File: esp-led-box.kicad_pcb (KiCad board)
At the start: 2 copper layers, 40 x 65 mm, 46 parts, among them J1 Conn_01x03, J2 Conn_01x03_Female, J3 Conn_01x02_Female, J4 USB_B_Micro, Q1 BSS138, SW3 SW_SPDT, U1 MP2307, U2 LM3940, U3 ESP-12F

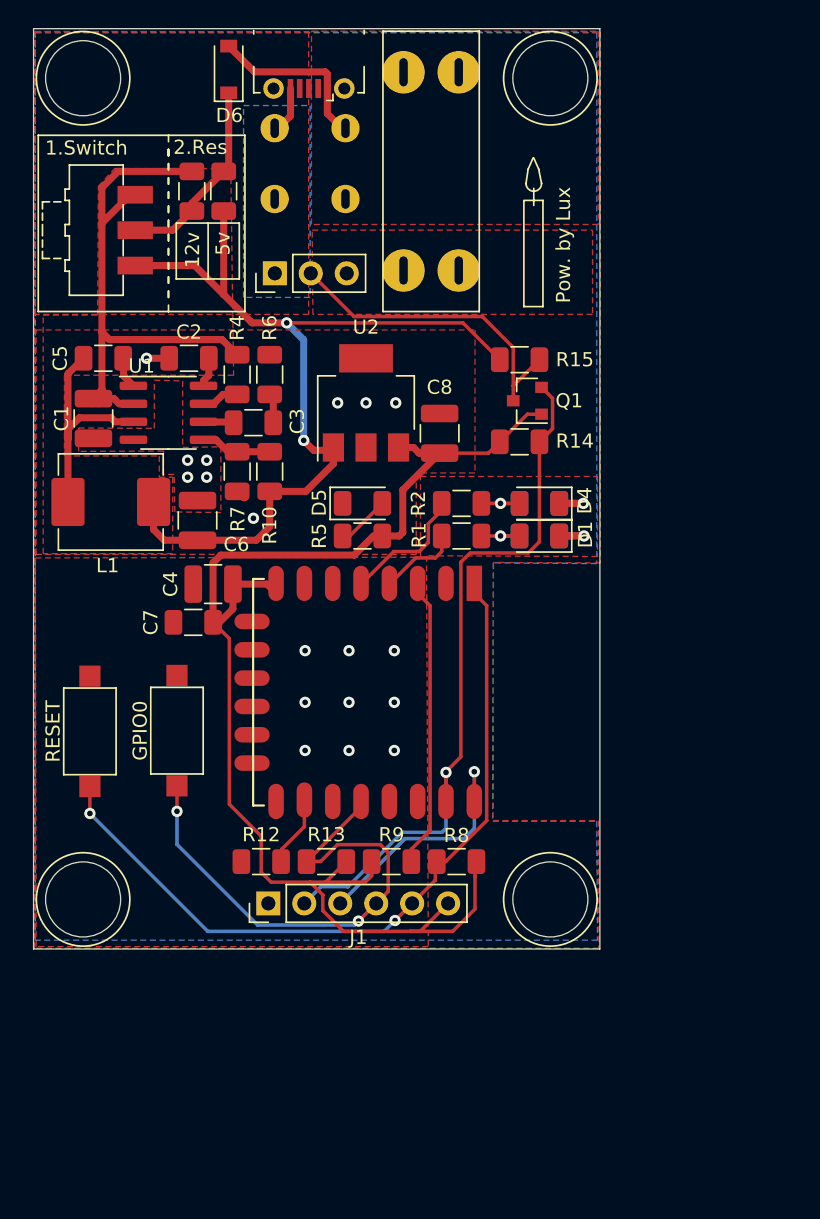
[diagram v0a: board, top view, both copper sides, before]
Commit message: my new version is coming
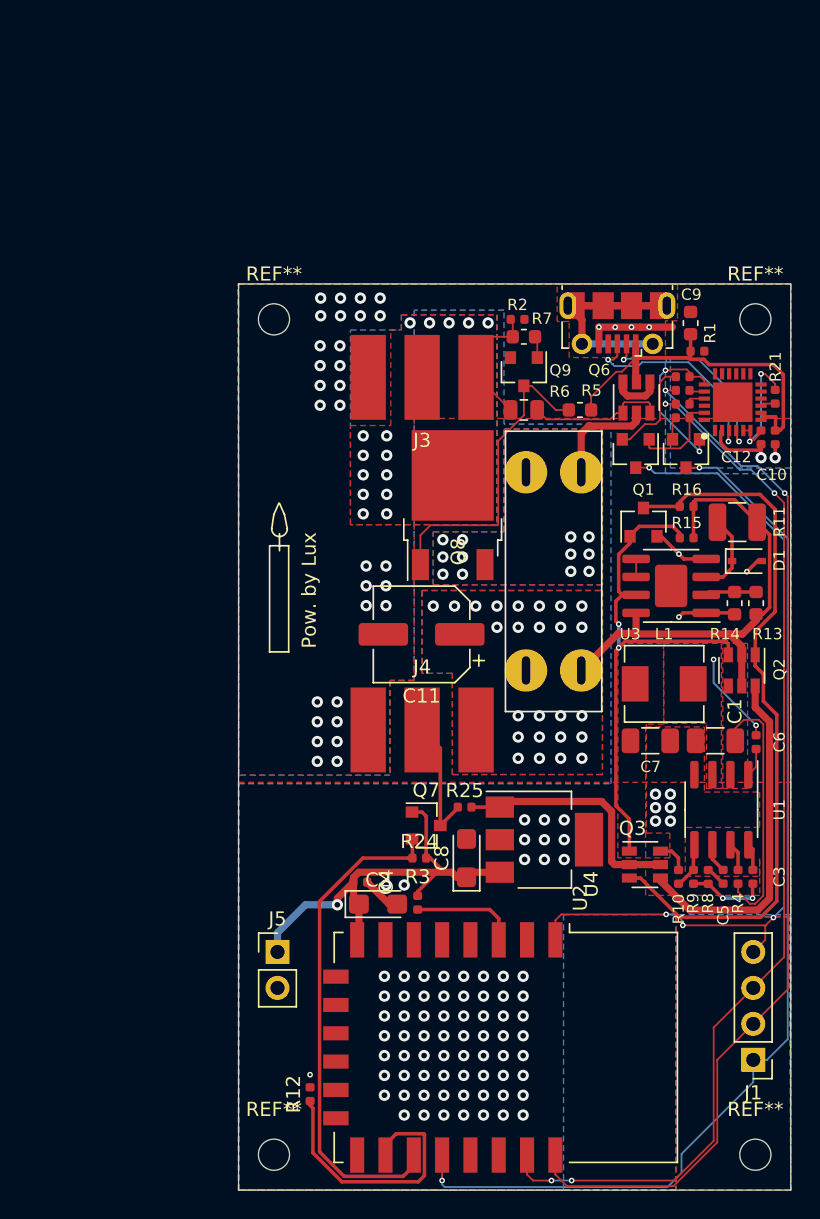
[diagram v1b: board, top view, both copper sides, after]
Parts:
- removed D2, D3, D4, D5: LED, LED_SMD:LED_1206_3216Metric
- removed D6: D, Diode_SMD:D_SOD-123
- removed GPIO0, RESET: SW_Push, Button_Switch_SMD:SW_SPST_CK_RS282G05A3
- removed the REF** at (147.5, 101.5)
- removed the REF** at (147.5, 43.5)
- removed the REF** at (114.5, 101.5)
- removed the REF** at (114.5, 43.5)
- removed SW3: SW_SPDT, Button_Switch_SMD:SW_SPDT_CK-JS102011SAQN
- added C10: 1uF, Capacitor_SMD:C_0402_1005Metric, F.Cu at (163.4, 68.8)
- added C11: 220u, Capacitor_SMD:CP_Elec_6.3x7.7, F.Cu at (138.4, 82.8)
- added C12: 100nF, Capacitor_SMD:C_0402_1005Metric, F.Cu at (162.4, 68.8)
- added C9: 10u, Capacitor_SMD:C_0603_1608Metric, F.Cu at (157.4, 60.8)
- added IC1: CP2105-F01-GMR, CP2105-F01-GMR:QFN50P400X400X80-25N-D, F.Cu at (160.4, 66.3)
- added J5: Conn_01x02, Connector_PinHeader_2.54mm:PinHeader_1x02_P2.54mm_Vertical, F.Cu at (128.2, 105.2)
- added Q2: Q_PMOS_DGS, Package_TO_SOT_SMD:SOT-23-6, F.Cu at (161.0, 85.3)
- added Q3: Q_PMOS_DGS, Package_TO_SOT_SMD:SOT-23-6, F.Cu at (154.2, 99.0)
- added Q4: S8050, Package_TO_SOT_SMD:SOT-23, F.Cu at (157.1, 70.0)
- added Q5: S8050, Package_TO_SOT_SMD:SOT-23, F.Cu at (153.6, 70.0)
- added Q6: Q_PMOS_DGS, Package_TO_SOT_SMD:SOT-23-6, F.Cu at (153.6, 66.0)
- added Q7: BSS138, Package_TO_SOT_SMD:SOT-23, F.Cu at (138.8, 96.2)
- added Q8: Q_PMOS_DGS, Package_TO_SOT_SMD:TO-252-2, F.Cu at (140.6, 73.6)
- added Q9: Q_NMOS, Package_TO_SOT_SMD:SOT-23, F.Cu at (145.7, 64.2)
- added R16: 20K, Resistor_SMD:R_0402_1005Metric, F.Cu at (157.1, 73.7)
- added R17: 12K, Resistor_SMD:R_0402_1005Metric, F.Cu at (156.9, 67.4)
- added R18: 12K, Resistor_SMD:R_0402_1005Metric, F.Cu at (156.9, 64.5)
- added R21: 4.7K, Resistor_SMD:R_0402_1005Metric, F.Cu at (163.4, 66.0)
- added R22: 300, Resistor_SMD:R_0402_1005Metric, F.Cu at (156.9, 66.5)
- added R23: 300, Resistor_SMD:R_0402_1005Metric, F.Cu at (156.9, 65.5)
- added R24: 10K, Resistor_SMD:R_0402_1005Metric, F.Cu at (138.3, 98.5)
- added R25: 10K, Resistor_SMD:R_0402_1005Metric, F.Cu at (141.5, 95.0)
- added REF**: MountingHole_2.2mm_M2, MountingHole:MountingHole_2.2mm_M2, F.Cu at (162.0, 60.5)
- added REF**: MountingHole_2.2mm_M2, MountingHole:MountingHole_2.2mm_M2, F.Cu at (128.0, 60.5)
- added REF**: MountingHole_2.2mm_M2, MountingHole:MountingHole_2.2mm_M2, F.Cu at (128.0, 119.5)
- added REF**: MountingHole_2.2mm_M2, MountingHole:MountingHole_2.2mm_M2, F.Cu at (162.0, 119.5)
- added U4: LM3940, Package_TO_SOT_SMD:SOT-223-3_TabPin2, F.Cu at (147.1, 97.2)
- C1: value 10uF/25V -> 10u/25V; footprint Capacitor_SMD:C_1210_3225Metric -> Capacitor_SMD:C_1206_3216Metric
- C2: value 0.1uF -> 10uF; footprint Capacitor_SMD:C_1206_3216Metric -> Capacitor_Tantalum_SMD:CP_EIA-3216-18_Kemet-A
- C3: value 3.9nF -> 100nF; footprint Capacitor_SMD:C_1206_3216Metric -> Capacitor_SMD:C_0402_1005Metric
- C4: value 10uF -> 100nF; footprint Capacitor_SMD:C_1210_3225Metric -> Capacitor_SMD:C_0402_1005Metric
- C5: value 10nF -> 3.9nF; footprint Capacitor_SMD:C_1206_3216Metric -> Capacitor_SMD:C_0402_1005Metric
- C6: value 22uF/6.3V -> 10nF; footprint Capacitor_SMD:C_1210_3225Metric -> Capacitor_SMD:C_0402_1005Metric
- C7: value 100nF -> 47uF/6.3V
- C8: footprint Capacitor_SMD:C_1210_3225Metric -> Capacitor_Tantalum_SMD:CP_EIA-3216-18_Kemet-A
- D1: value LED -> 2.4V; footprint LED_SMD:LED_1206_3216Metric -> Diode_SMD:D_SOD-323
- J1: value Conn_01x03 -> Conn_01x04; footprint Connector_PinHeader_2.54mm:PinHeader_1x06_P2.54mm_Vertical -> Connector_PinHeader_2.54mm:PinHeader_1x04_P2.54mm_Vertical
- J2: value Conn_01x03_Female -> USB_B_Micro; footprint Connector_PinHeader_2.54mm:PinHeader_1x03_P2.54mm_Vertical -> Connector_USB:USB_Micro-B_Molex-105017-0001
- J3: value Conn_01x02_Female -> Conn_01x03_Female; footprint esp-light-box:WG235-2P -> esp-light-box:SolderWire_1x03_2.5x6; moved to F.Cu
- J4: value USB_B_Micro -> Conn_01x03_Female; footprint Connector_USB:USB_Micro-B_Molex-105017-0001 -> esp-light-box:SolderWire_1x03_2.5x6
- L1: footprint Inductor_SMD:L_Abracon_ASPI-0630LR -> Inductor_SMD:L_Sunlord_MWSA0518_5.4x5.2mm
- Q1: value BSS138 -> Q_NMOS
- R1, R2: value 120 -> 1M; footprint Resistor_SMD:R_1206_3216Metric -> Resistor_SMD:R_0402_1005Metric
- R10, R12, R4: footprint Resistor_SMD:R_1206_3216Metric -> Resistor_SMD:R_0402_1005Metric
- R11: value 0 -> 360; footprint Resistor_SMD:R_1206_3216Metric -> Resistor_SMD:R_1210_3225Metric
- R13: value 10K -> 24K; footprint Resistor_SMD:R_1206_3216Metric -> Resistor_SMD:R_0603_1608Metric
- R14: footprint Resistor_SMD:R_1206_3216Metric -> Resistor_SMD:R_0603_1608Metric
- R15: value 10K -> 20K; footprint Resistor_SMD:R_1206_3216Metric -> Resistor_SMD:R_0402_1005Metric
- R3: value 0 -> 10K; footprint Resistor_SMD:R_1206_3216Metric -> Resistor_SMD:R_0402_1005Metric
- R5: value 120 -> 20K; footprint Resistor_SMD:R_1206_3216Metric -> Resistor_SMD:R_0603_1608Metric
- R6: value 6.8K -> 300; footprint Resistor_SMD:R_1206_3216Metric -> Resistor_SMD:R_0805_2012Metric
- R7: value 10K/1% -> 20K; footprint Resistor_SMD:R_1206_3216Metric -> Resistor_SMD:R_0603_1608Metric
- R8: value 10K -> 6.8K; footprint Resistor_SMD:R_1206_3216Metric -> Resistor_SMD:R_0402_1005Metric
- R9: value 10K -> 10K/1%; footprint Resistor_SMD:R_1206_3216Metric -> Resistor_SMD:R_0402_1005Metric
- U2: value LM3940 -> ESP-12F; footprint Package_TO_SOT_SMD:SOT-223-3_TabPin2 -> RF_Module:ESP-12E
- U3: value ESP-12F -> LM211; footprint ESP8266:ESP-12E -> Package_SO:SOIC-8-1EP_3.9x4.9mm_P1.27mm_EP2.29x3mm
- moved C5 57.1 mm to (159.7, 99.9), turned to 270 degrees
- moved R3 52.7 mm to (138.2, 101.7), turned to 270 degrees
- moved R4 50.1 mm to (160.8, 99.9), turned to 90 degrees
- moved C1 49.5 mm to (159.2, 90.3), turned to 180 degrees
- moved U1 48.1 mm to (159.6, 95.1), turned to 270 degrees
- moved C3 47.7 mm to (161.8, 99.9), turned to 270 degrees
- moved J4 47.4 mm to (138.5, 89.5), turned to 0 degrees
- moved U2 46.6 mm to (144.4, 111.9), turned to 270 degrees
- moved R11 43.2 mm to (160.7, 74.8), turned to 0 degrees
- moved C6 42.4 mm to (162.1, 90.4), turned to 270 degrees
- moved L1 41.1 mm to (155.6, 86.2), turned to 180 degrees
- moved C2 40.8 mm to (135.3, 101.8), turned to 0 degrees
- moved R10 40.7 mm to (156.6, 99.9), turned to 270 degrees
- moved J1 36.0 mm to (161.8, 112.8), turned to 180 degrees
- moved R13 35.4 mm to (162.1, 80.5), turned to 90 degrees
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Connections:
- C2 pad 1: Net-(C2-Pad1) -> +3V3
- C3 pad 2: Net-(C3-Pad2) -> GND
- C6 pad 1: +5V -> Net-(C6-Pad1)
- C6 pad 2: GND -> Net-(C6-Pad2)
- C7 pad 1: +3V3 -> /BUCK_5V
- D1 pad 1: GND -> Net-(D1-Pad1)
- D1 pad 2: Net-(D1-Pad2) -> GND
- F1 pad 1: Net-(F1-Pad1) -> /DC_VDD
- F1 pad 2: VSS -> VDD
- J1 pad 1: GND -> /GPIO0
- J1 pad 2: /RXD|CONTROL -> /TXD
- J1 pad 3: /TXD -> /RXD
- J1 pad 4: /GPIO0 -> /RESET
- J2 pad 1: GND -> VBUS
- J2 pad 2: Net-(J2-Pad2) -> /D-
- J2 pad 3: Net-(F1-Pad1) -> /D+
- J3 pad 1: GND -> VDC
- J3 pad 2: VSS -> VDC
- J4 pad 1: VSS -> GND
- J4 pad 3: Net-(J4-Pad3) -> VDD
- L1 pad 1: Net-(C5-Pad1) -> Net-(C6-Pad1)
- L1 pad 2: +5V -> /BUCK_5V
- Q1 pad 1: +3V3 -> /~12V_SEL
- Q1 pad 2: /RXD|CONTROL -> GND
- Q1 pad 3: Net-(J2-Pad2) -> /~5V_SEL
- R1 pad 1: /GREEN_LED -> VBUS
- R1 pad 2: Net-(D1-Pad2) -> GND
- R10 pad 1: +5V -> /BUCK_5V
- R11 pad 1: +VDC -> Net-(D1-Pad1)
- R11 pad 2: +5V -> VDD
- R12 pad 1: GND -> Net-(R12-Pad1)
- R12 pad 2: Net-(R12-Pad2) -> GND
- R13 pad 1: +3V3 -> VDD
- R13 pad 2: /GPIO0 -> Net-(R13-Pad2)
- R14 pad 1: /RXD|CONTROL -> Net-(R13-Pad2)
- R14 pad 2: +3V3 -> GND
- R15 pad 1: Net-(J2-Pad2) -> VDD
- R15 pad 2: +5V -> /~12V_SEL
- R2 pad 1: /RED_LED -> VDC
- R2 pad 2: Net-(D3-Pad2) -> GND
- R3 pad 1: +VDC -> +3V3
- R3 pad 2: +12V -> Net-(R3-Pad2)
- R5 pad 1: +3V3 -> VBUS
- R5 pad 2: Net-(D5-Pad2) -> /~VDC_SEL
- R6 pad 1: Net-(C3-Pad2) -> VDC
- R6 pad 2: GND -> /VDC_ON
- R7 pad 1: Net-(R10-Pad2) -> VDC
- R7 pad 2: GND -> Net-(Q9-Pad1)
- R8 pad 1: /RESET -> Net-(C5-Pad2)
- R8 pad 2: +3V3 -> GND
- R9 pad 1: Net-(R9-Pad1) -> Net-(R10-Pad2)
- R9 pad 2: +3V3 -> GND
- U1 pad 1: Net-(C5-Pad2) -> Net-(C6-Pad2)
- U1 pad 3: Net-(C5-Pad1) -> Net-(C6-Pad1)
- U1 pad 6: Net-(C3-Pad1) -> Net-(C5-Pad1)
- U1 pad 8: Net-(C2-Pad1) -> Net-(C3-Pad1)
- U2 pad 1: +5V -> /RESET
- U2 pad 2: GND -> Net-(U2-Pad2)
- U2 pad 3: +3V3 -> Net-(R3-Pad2)
- U3 pad 1: /RESET -> GND
- U3 pad 2: Net-(U3-Pad2) -> Net-(R13-Pad2)
- U3 pad 3: Net-(R9-Pad1) -> Net-(D1-Pad1)
- U3 pad 4: /GREEN_LED -> GND
- U3 pad 5: /RED_LED -> Net-(U3-Pad5)
- U3 pad 6: Net-(U3-Pad6) -> Net-(U3-Pad5)
- U3 pad 7: Net-(U3-Pad7) -> /~12V_SEL
- U3 pad 8: +3V3 -> VDD
- U3 pad 9: GND -> (no net)
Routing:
- net /RXD: track 0.00 -> 76.9 mm, vias 0 -> 4
- net +3V3: track 95.5 -> 33.5 mm, vias 0 -> 1
- net /TXD: track 17.1 -> 74.6 mm, vias 1 -> 2
- net /RXD|CONTROL: track 52.2 -> 0.00 mm, vias 1 -> 0
- net /~5V_SEL: track 0.00 -> 51.2 mm
- net +5V: track 65.5 -> 17.4 mm, vias 2 -> 0
- net /GPIO0: track 39.3 -> 77.2 mm
- net /~12V_SEL: track 0.00 -> 37.5 mm, vias 0 -> 2
- net /LED_CTRL: track 0.00 -> 35.3 mm
- net VDD: track 0.00 -> 35.2 mm, vias 0 -> 25
- net VBUS: track 0.00 -> 30.4 mm
- net /DC_5V: track 0.00 -> 24.5 mm
- net Net-(J2-Pad2): track 22.8 -> 0.00 mm
- net +12V: track 40.9 -> 18.3 mm
- net /~VDC_SEL: track 0.00 -> 22.3 mm
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- added copper zone on B.Cu, net (none)
- added copper zone on F.Cu, net +12V
- added copper zone on F.Cu, net /BUCK_5V
- added copper zone on B.Cu, net /DC_VDD
- added copper zone on F.Cu, net /DC_VDD
- added copper zone on F.Cu, net Net-(C6-Pad1)
- added copper zone on B.Cu, net VDC
- added copper zone on F.Cu, net VDC
- added copper zone on B.Cu, net VDD
- added copper zone on F.Cu, net VDD
- removed copper zone on F.Cu, net Net-(F1-Pad1)
- removed copper zone on F.Cu, net VSS
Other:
- board size 40 x 65 mm -> 39 x 64 mm
- net class Default: clearance 0.2 -> 0.127; trace_width 0.25 -> 0.127
- net class Digital Power added: clearance 0.127, trace_width 0.254, via_dia 0.8, via_drill 0.4
- net class Signal added: clearance 0.127, trace_width 0.254, via_dia 0.8, via_drill 0.4
- rule trace_clearance: 0.2 -> 0.127
- rule trace_min: 0.2 -> 0.127
- rule via_min_drill: 0.3 -> 0.2
- board text removed: "1.Switch"
- board text removed: "12v"
- board text removed: "2.Res"
- board text removed: "5v"
